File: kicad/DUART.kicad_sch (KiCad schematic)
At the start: 8 parts, among them J6 PORTA serial, J7 PORTB serial, J8 DUART I/O, U15 68681

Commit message: saved again
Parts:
- C19, C20, C7: footprint Capacitor_THT:CP_Radial_D5.0mm_P2.50mm -> Capacitor_THT:C_Disc_D5.0mm_W2.5mm_P2.50mm
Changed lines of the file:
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@@
       (effects (font (size 1.27 1.27)))
     )
-    (property "Footprint" "Capacitor_THT:CP_Radial_D5.0mm_P2.50mm" (at 94.9452 36.83 0)
+    (property "Footprint" "Capacitor_THT:C_Disc_D5.0mm_W2.5mm_P2.50mm" (at 94.9452 36.83 0)
       (effects (font (size 1.27 1.27)) hide)
     )
@@
       (effects (font (size 1.27 1.27)) (justify left))
     )
-    (property "Footprint" "Capacitor_THT:CP_Radial_D5.0mm_P2.50mm" (at 185.1152 124.46 0)
+    (property "Footprint" "Capacitor_THT:C_Disc_D5.0mm_W2.5mm_P2.50mm" (at 185.1152 124.46 0)
       (effects (font (size 1.27 1.27)) hide)
     )
@@
       (effects (font (size 1.27 1.27)) (justify left))
     )
-    (property "Footprint" "Capacitor_THT:CP_Radial_D5.0mm_P2.50mm" (at 105.1052 36.83 0)
-      (effects (font (size 1.27 1.27)) hide)
-    )
+    (property "Footprint" "Capacitor_THT:C_Disc_D5.0mm_W2.5mm_P2.50mm" (at 105.1052 36.83 0)
+      (effects (font (size 1.27 1.27)) hide)
+    )

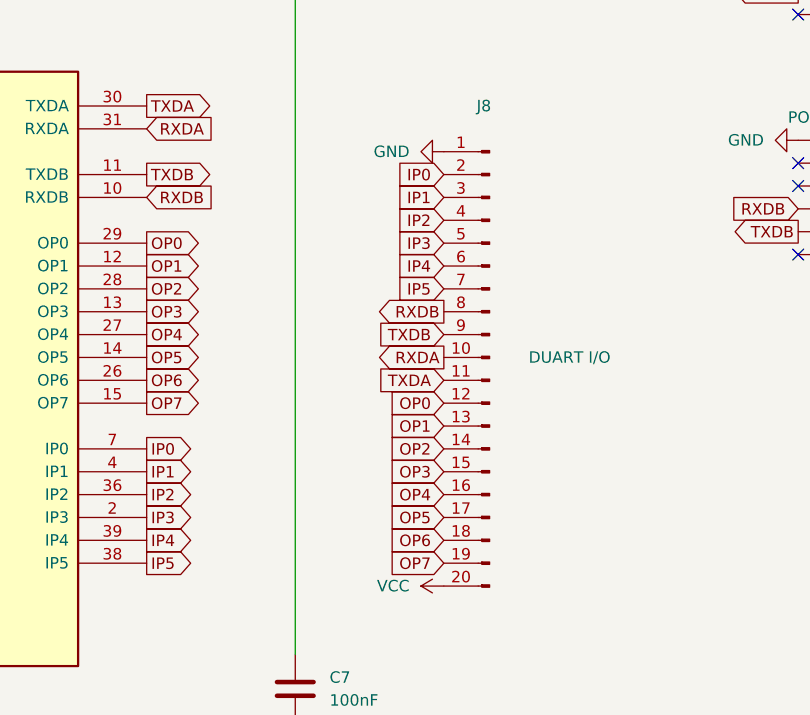
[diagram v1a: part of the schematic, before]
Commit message: fiddlign with placement
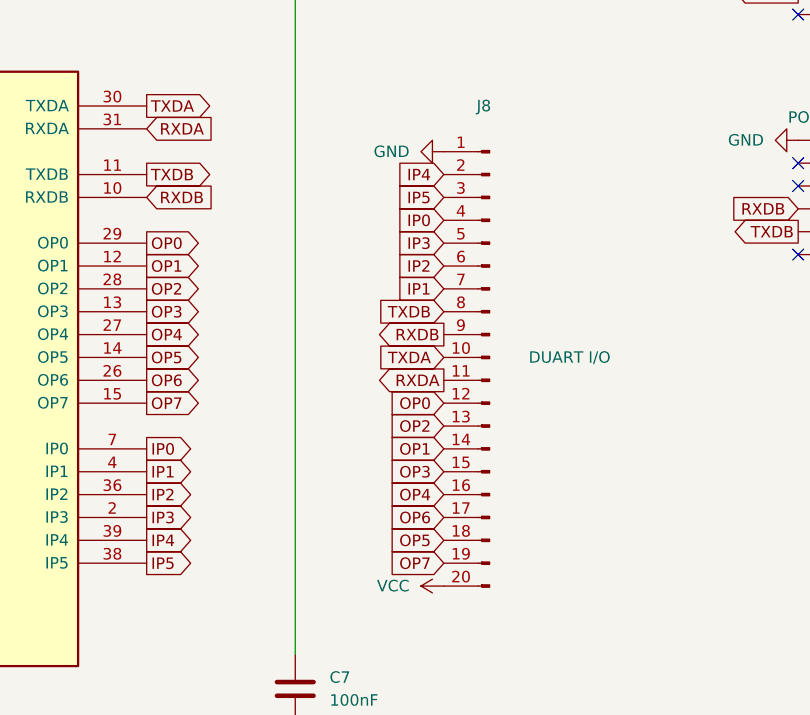
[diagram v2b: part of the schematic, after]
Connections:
- net IP0: now also J8.4 (Pin_4); no longer J8.2 (Pin_2)
- net IP1: now also J8.7 (Pin_7); no longer J8.3 (Pin_3)
- net IP2: now also J8.6 (Pin_6); no longer J8.4 (Pin_4)
- net IP4: now also J8.2 (Pin_2); no longer J8.6 (Pin_6)
- net IP5: now also J8.3 (Pin_3); no longer J8.7 (Pin_7)
- net OP1: now also J8.14 (Pin_14); no longer J8.13 (Pin_13)
- net OP2: now also J8.13 (Pin_13); no longer J8.14 (Pin_14)
- net OP5: now also J8.18 (Pin_18); no longer J8.17 (Pin_17)
- net OP6: now also J8.17 (Pin_17); no longer J8.18 (Pin_18)
- net RXDA: now also J8.11 (Pin_11); no longer J8.10 (Pin_10)
- net RXDB: now also J8.9 (Pin_9); no longer J8.8 (Pin_8)
- net TXDA: now also J8.10 (Pin_10); no longer J8.11 (Pin_11)
- net TXDB: now also J8.8 (Pin_8); no longer J8.9 (Pin_9)

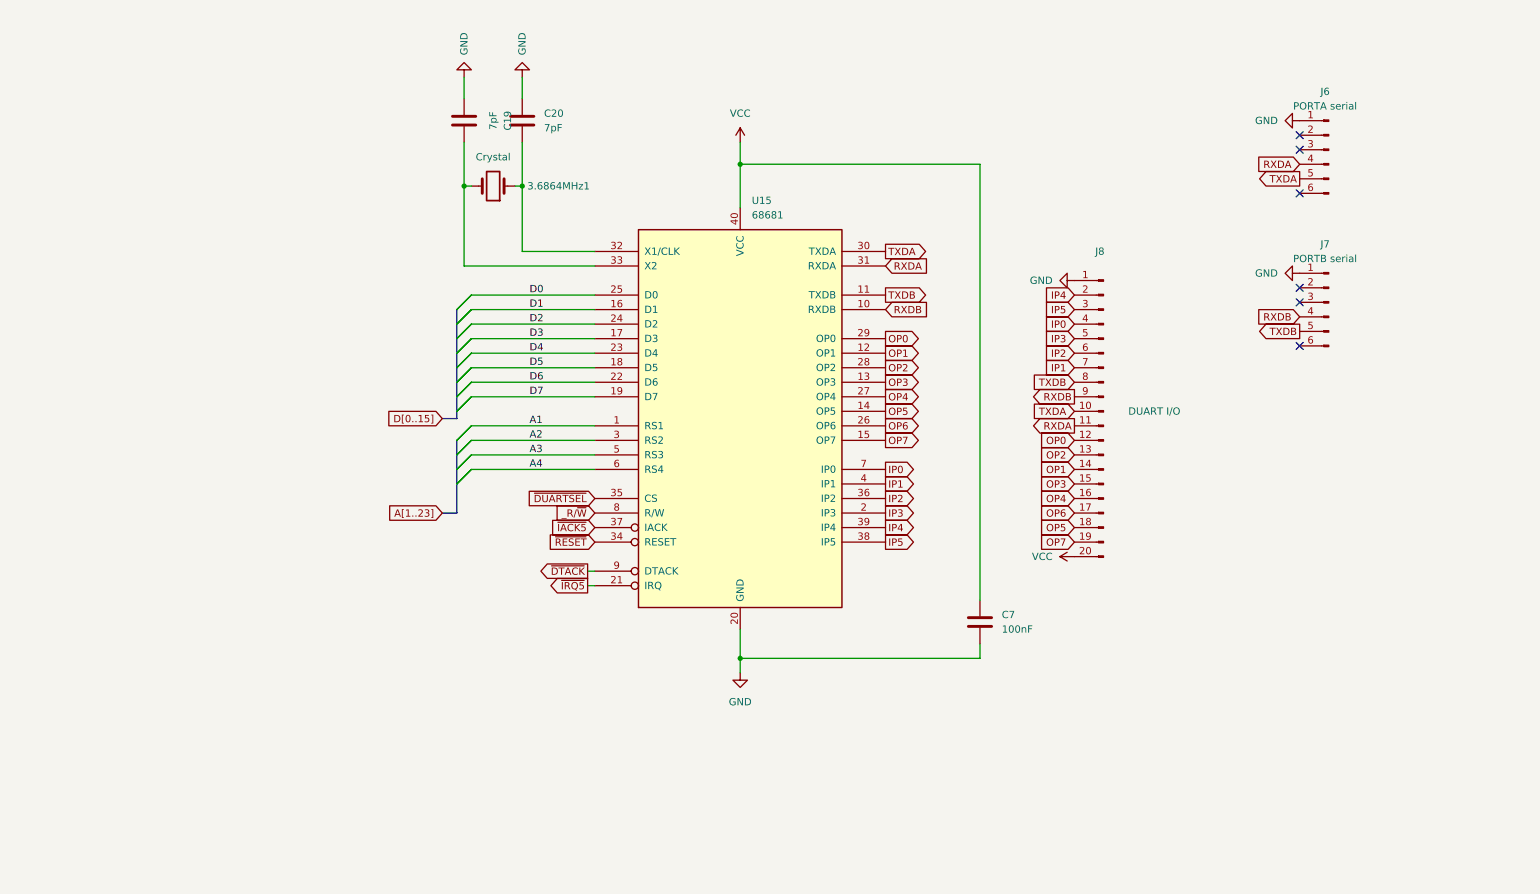
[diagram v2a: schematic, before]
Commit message: got irq to work
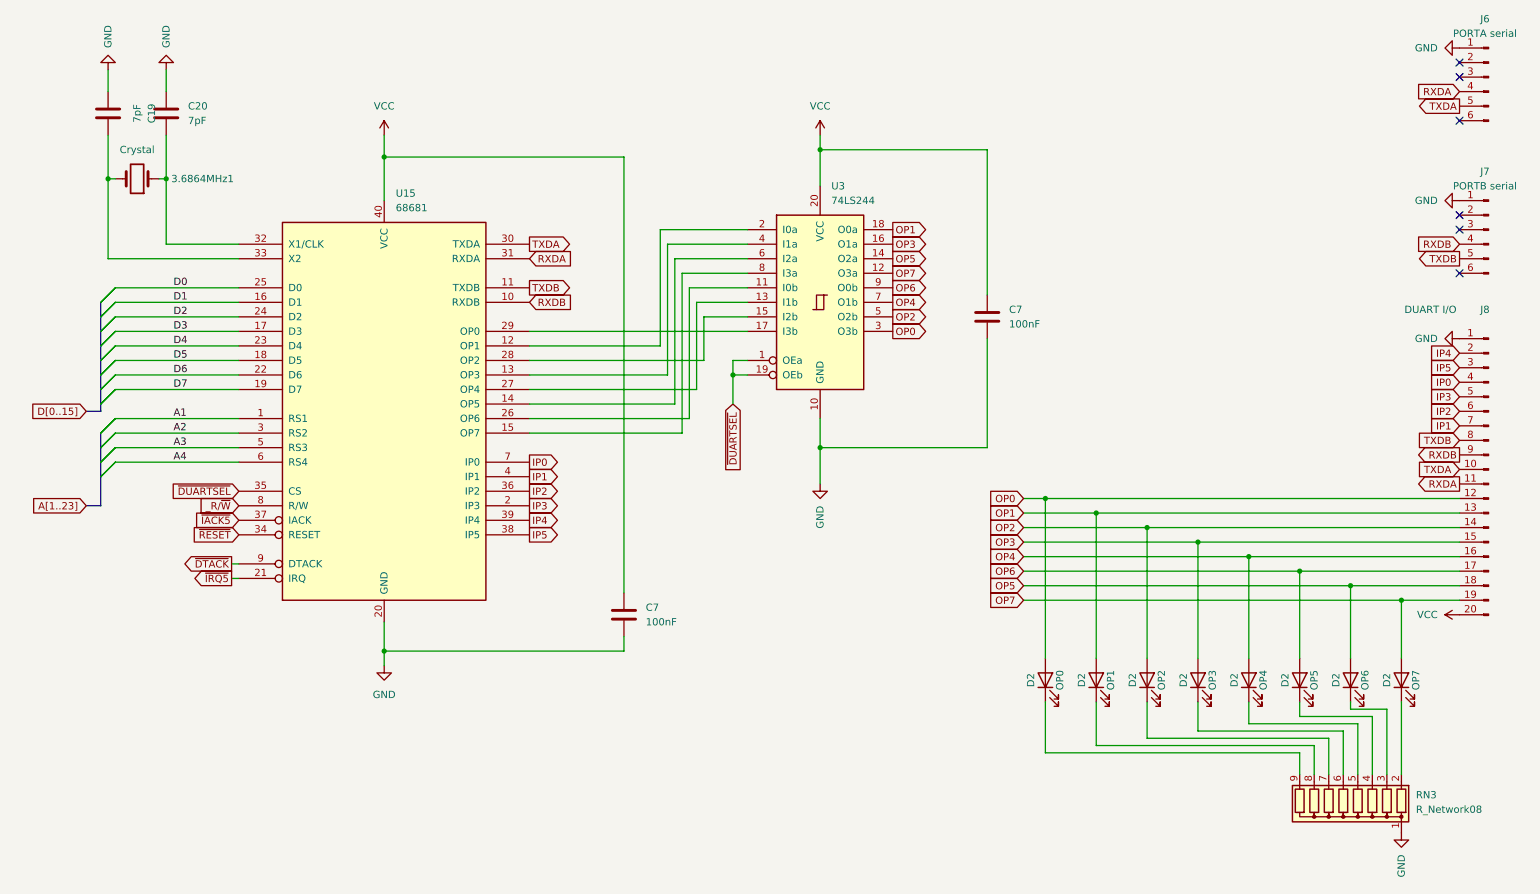
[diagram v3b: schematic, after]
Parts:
- added C7: 100nF, Capacitor_THT:C_Disc_D5.0mm_W2.5mm_P2.50mm, symbol Device:C
- added D2: OP4, LED_THT:LED_D5.0mm, symbol Device:LED
- added D2: OP2, LED_THT:LED_D5.0mm, symbol Device:LED
- added D2: OP3, LED_THT:LED_D5.0mm, symbol Device:LED
- added D2: OP5, LED_THT:LED_D5.0mm, symbol Device:LED
- added D2: OP7, LED_THT:LED_D5.0mm, symbol Device:LED
- added D2: OP6, LED_THT:LED_D5.0mm, symbol Device:LED
- added D2: OP0, LED_THT:LED_D5.0mm, symbol Device:LED
- added D2: OP1, LED_THT:LED_D5.0mm, symbol Device:LED
- added RN3: R_Network08, Resistor_THT:R_Array_SIP9, symbol Device:R_Network08
- added U3: 74LS244, Package_DIP:DIP-20_W7.62mm, symbol 74xx:74LS244
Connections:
- net GND: now also C7.2, RN3.1 (common), U3.10 (GND)
- net OP0: now also D2.2 (A), U3.3 (O3b); no longer U15.29 (OP0)
- net OP1: now also J8.13 (Pin_13), D2.2 (A), U3.18 (O0a); no longer J8.14 (Pin_14), U15.12 (OP1)
- net OP2: now also J8.14 (Pin_14), D2.2 (A), U3.5 (O2b); no longer J8.13 (Pin_13), U15.28 (OP2)
- net OP3: now also D2.2 (A), U3.16 (O1a); no longer U15.13 (OP3)
- net OP4: now also D2.2 (A), U3.7 (O1b); no longer U15.27 (OP4)
- net OP5: now also D2.2 (A), U3.14 (O2a); no longer U15.14 (OP5)
- net OP6: now also D2.2 (A), U3.9 (O0b); no longer U15.26 (OP6)
- net OP7: now also D2.2 (A), U3.12 (O3a); no longer U15.15 (OP7)
- net VCC: now also C7.1, U3.20 (VCC)
- net ~{DUARTSEL}: now also U3.1 (OEa), U3.19 (OEb)
- new net: U15.26 (OP6), U3.11 (I0b)
- new net: U15.27 (OP4), U3.13 (I1b)
- new net: U15.28 (OP2), U3.15 (I2b)
- new net: U15.29 (OP0), U3.17 (I3b)
- new net: U15.12 (OP1), U3.2 (I0a)
- new net: U15.13 (OP3), U3.4 (I1a)
- new net: U15.14 (OP5), U3.6 (I2a)
- new net: U15.15 (OP7), U3.8 (I3a)
- new net: D2.1 (K), RN3.5 (R4)
- new net: D2.1 (K), RN3.7 (R6)
- new net: D2.1 (K), RN3.6 (R5)
- new net: D2.1 (K), RN3.2 (R1)
- new net: D2.1 (K), RN3.3 (R2)
- new net: D2.1 (K), RN3.4 (R3)
- new net: D2.1 (K), RN3.8 (R7)
- new net: D2.1 (K), RN3.9 (R8)
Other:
- moved on the sheet: 3.6864MHz1, C19, C20, C7, J6, J7, J8, U15
